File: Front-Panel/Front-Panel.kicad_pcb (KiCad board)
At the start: 2 copper layers, 20 x 128.5 mm, 0 parts

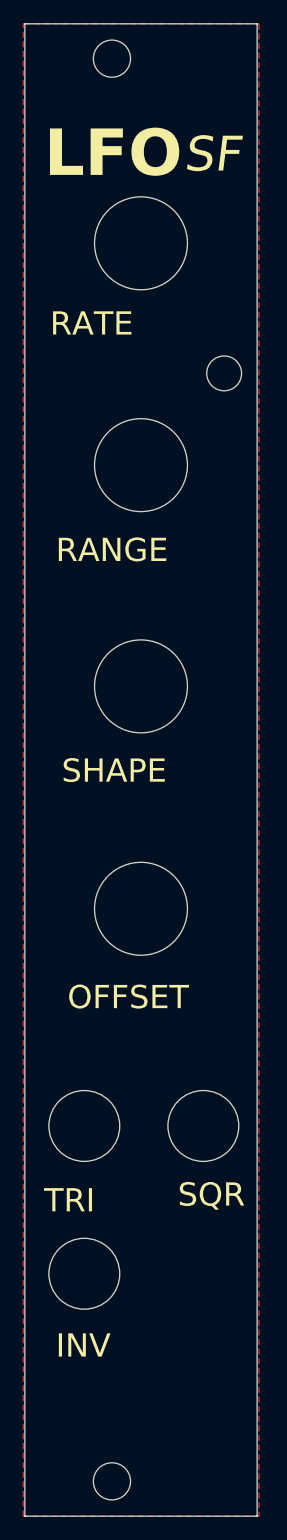
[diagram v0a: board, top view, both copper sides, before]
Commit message: review and update
Reviewed ad updated board dimensions and outlines. Checked position of jacks and pots.
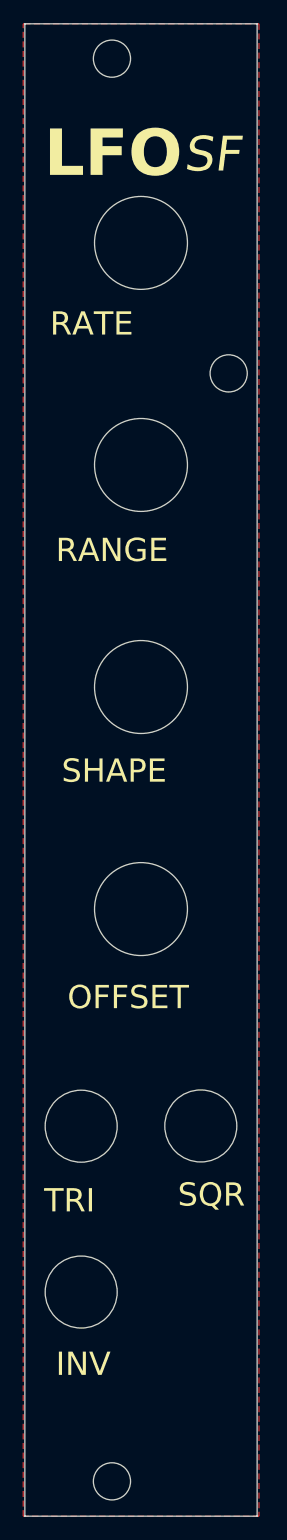
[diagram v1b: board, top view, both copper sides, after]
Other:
- outline, holes or cut-outs redrawn
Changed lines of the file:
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@@
 	)
 	(gr_line
-		(start 66.5 127.625)
-		(end 122.5 127.625)
+		(start 66.5 129.199999)
+		(end 122.5 129.199999)
 		(stroke
 			(width 0.1)
@@
 	)
 	(gr_circle
-		(center 83.96 114.9)
-		(end 87.009999 114.9)
-		(stroke
-			(width 0.1)
-			(type default)
-		)
-		(fill no)
-		(layer "Edge.Cuts")
-	)
-	(gr_circle
-		(center 83.96 127.625)
-		(end 87.009999 127.625)
+		(center 83.69 114.92)
+		(end 86.789999 114.92)
+		(stroke
+			(width 0.1)
+			(type default)
+		)
+		(fill no)
+		(layer "Edge.Cuts")
+	)
+	(gr_circle
+		(center 83.69 129.199999)
+		(end 86.789999 129.199999)
 		(stroke
 			(width 0.1)
@@
 	)
 	(gr_circle
-		(center 88.84 38.9)
-		(end 92.84 38.9)
-		(stroke
-			(width 0.1)
-			(type default)
-		)
-		(fill no)
-		(layer "Edge.Cuts")
-	)
-	(gr_circle
-		(center 88.84 58)
-		(end 92.84 58)
-		(stroke
-			(width 0.1)
-			(type default)
-		)
-		(fill no)
-		(layer "Edge.Cuts")
-	)
-	(gr_circle
-		(center 88.84 77.05)
-		(end 92.84 77.05)
-		(stroke
-			(width 0.1)
-			(type default)
-		)
-		(fill no)
-		(layer "Edge.Cuts")
-	)
-	(gr_circle
-		(center 88.84 96.2)
-		(end 92.84 96.2)
-		(stroke
-			(width 0.1)
-			(type default)
-		)
-		(fill no)
-		(layer "Edge.Cuts")
-	)
-	(gr_circle
-		(center 94.21 114.9)
-		(end 97.259999 114.9)
-		(stroke
-			(width 0.1)
-			(type default)
-		)
-		(fill no)
-		(layer "Edge.Cuts")
-	)
-	(gr_circle
-		(center 96 50.1)
-		(end 97.5 50.1)
+		(center 88.84 38.865)
+		(end 92.84 38.865)
+		(stroke
+			(width 0.1)
+			(type default)
+		)
+		(fill no)
+		(layer "Edge.Cuts")
+	)
+	(gr_circle
+		(center 88.84 57.985)
+		(end 92.84 57.985)
+		(stroke
+			(width 0.1)
+			(type default)
+		)
+		(fill no)
+		(layer "Edge.Cuts")
+	)
+	(gr_circle
+		(center 88.84 77.105)
+		(end 92.84 77.105)
+		(stroke
+			(width 0.1)
+			(type default)
+		)
+		(fill no)
+		(layer "Edge.Cuts")
+	)
+	(gr_circle
+		(center 88.84 96.225)
+		(end 92.84 96.225)
+		(stroke
+			(width 0.1)
+			(type default)
+		)
+		(fill no)
+		(layer "Edge.Cuts")
+	)
+	(gr_circle
+		(center 93.99 114.9)
+		(end 97.089999 114.9)
+		(stroke
+			(width 0.1)
+			(type default)
+		)
+		(fill no)
+		(layer "Edge.Cuts")
+	)
+	(gr_circle
+		(center 96.39 50.099999)
+		(end 97.99 50.099999)
 		(stroke
 			(width 0.1)
@@
 	)
 	(gr_text "INV"
-		(at 81.5 135 0)
+		(at 81.5 136.574999 0)
 		(layer "F.SilkS")
 		(effects
@@
 			(polygon
 				(pts
-					(xy 81.729588 132.659162) (xy 81.729588 134.66) (xy 81.995568 134.66) (xy 81.995568 132.659162)
-				)
-			)
-			(polygon
-				(pts
-					(xy 82.440457 132.659162) (xy 82.440457 134.66) (xy 82.692515 134.66) (xy 82.692515 133.054225)
-					(xy 82.698133 133.054225) (xy 83.742515 134.66) (xy 84.033653 134.66) (xy 84.033653 132.659162)
-					(xy 83.781716 132.659162) (xy 83.781716 134.281667) (xy 83.776099 134.281667) (xy 82.72329 132.659162)
-				)
-			)
-			(polygon
-				(pts
-					(xy 85.250471 134.66) (xy 85.961706 132.659162) (xy 85.68449 132.659162) (xy 85.107711 134.393775)
-					(xy 85.102093 134.393775) (xy 84.530931 132.659162) (xy 84.245289 132.659162) (xy 84.948098 134.66)
-				)
-			)
+					(xy 81.729588 134.234161) (xy 81.729588 136.234999) (xy 81.995568 136.234999) (xy 81.995568 134.234161)
+				)
+			)
+			(polygon
+				(pts
+					(xy 82.440457 134.234161) (xy 82.440457 136.234999) (xy 82.692515 136.234999) (xy 82.692515 134.629224)
+					(xy 82.698133 134.629224) (xy 83.742515 136.234999) (xy 84.033653 136.234999) (xy 84.033653 134.234161)
+					(xy 83.781716 134.234161) (xy 83.781716 135.856666) (xy 83.776099 135.856666) (xy 82.72329 134.234161)
+				)
+			)
+			(polygon
+				(pts
+					(xy 85.250471 136.234999) (xy 85.961706 134.234161) (xy 85.68449 134.234161) (xy 85.107711 135.968774)
+					(xy 85.102093 135.968774) (xy 84.530931 134.234161) (xy 84.245289 134.234161) (xy 84.948098 136.234999)
+				)
+			)
